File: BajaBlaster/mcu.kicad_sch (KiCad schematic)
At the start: 15 parts, among them J1 Conn_01x06_Socket, SW1 SW_Push, SW2 SW_Push, U1 ESP32-WROOM-32, U2 MPU-6050

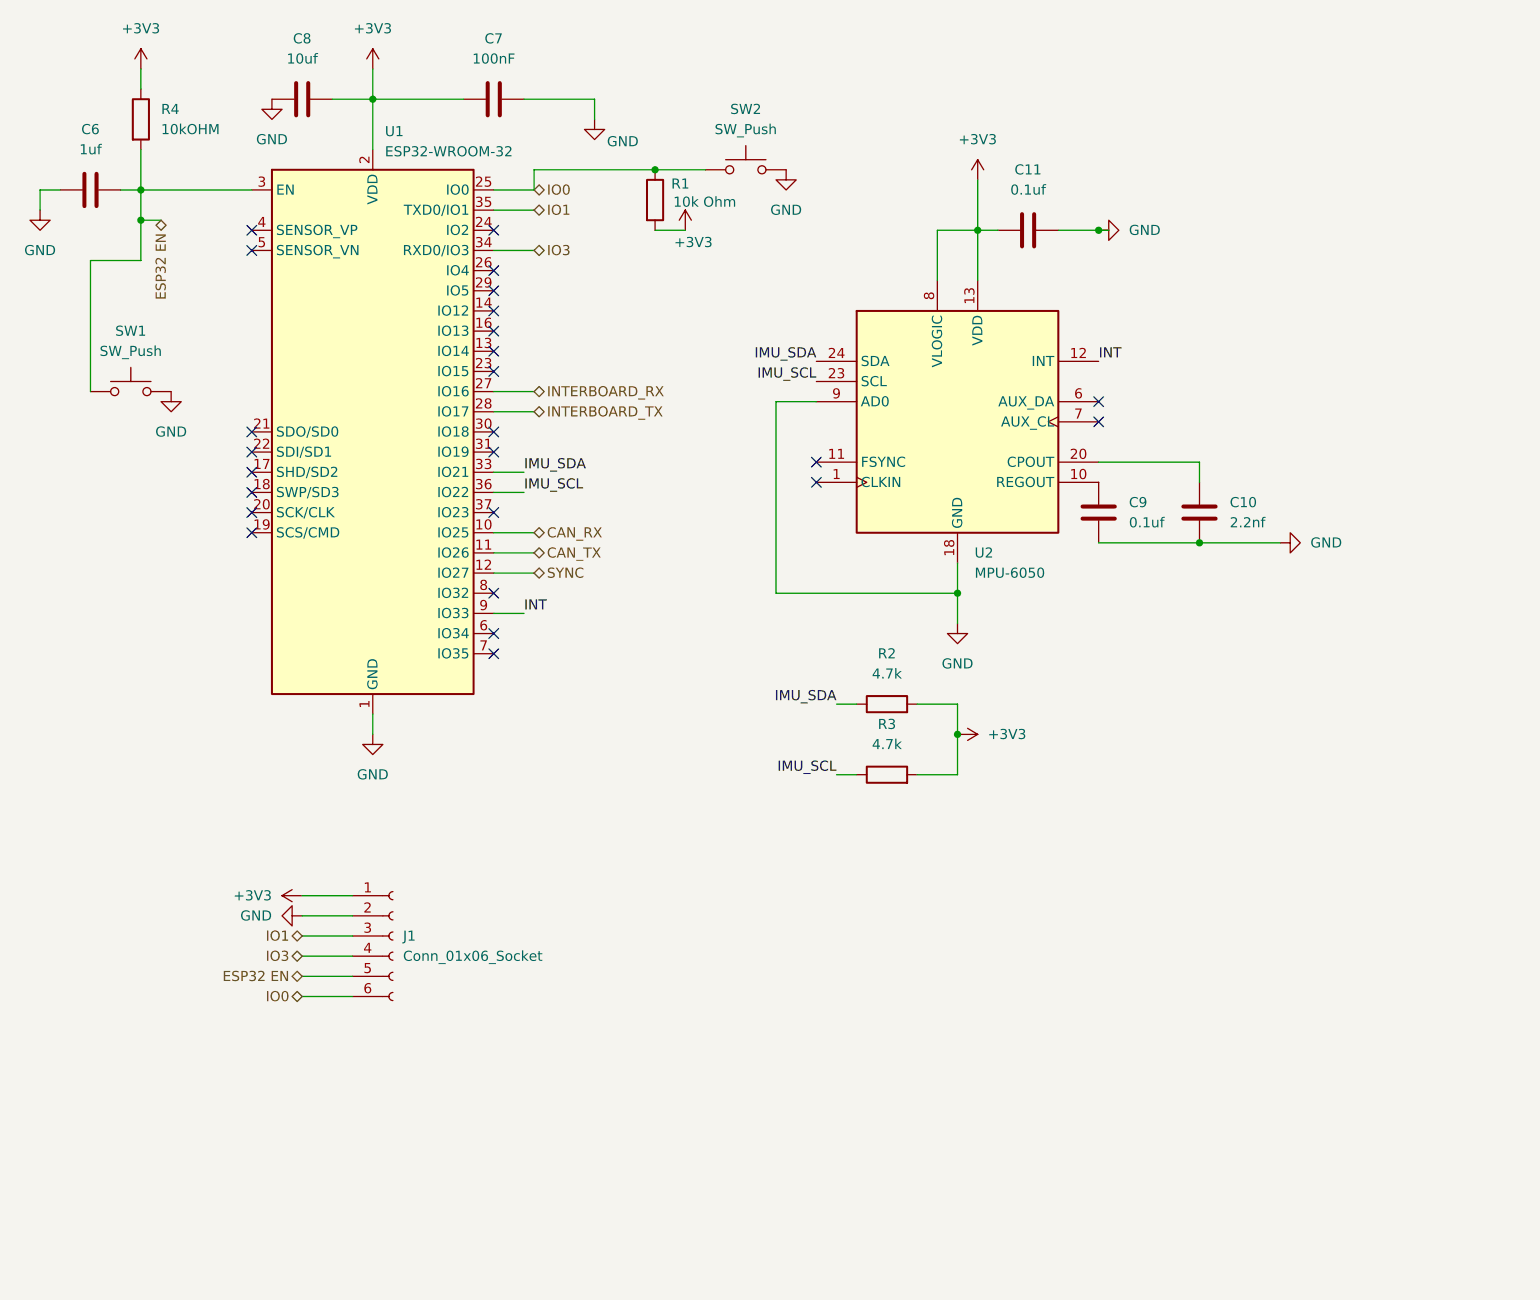
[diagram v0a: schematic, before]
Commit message: doing lots of small tweaks and fixups
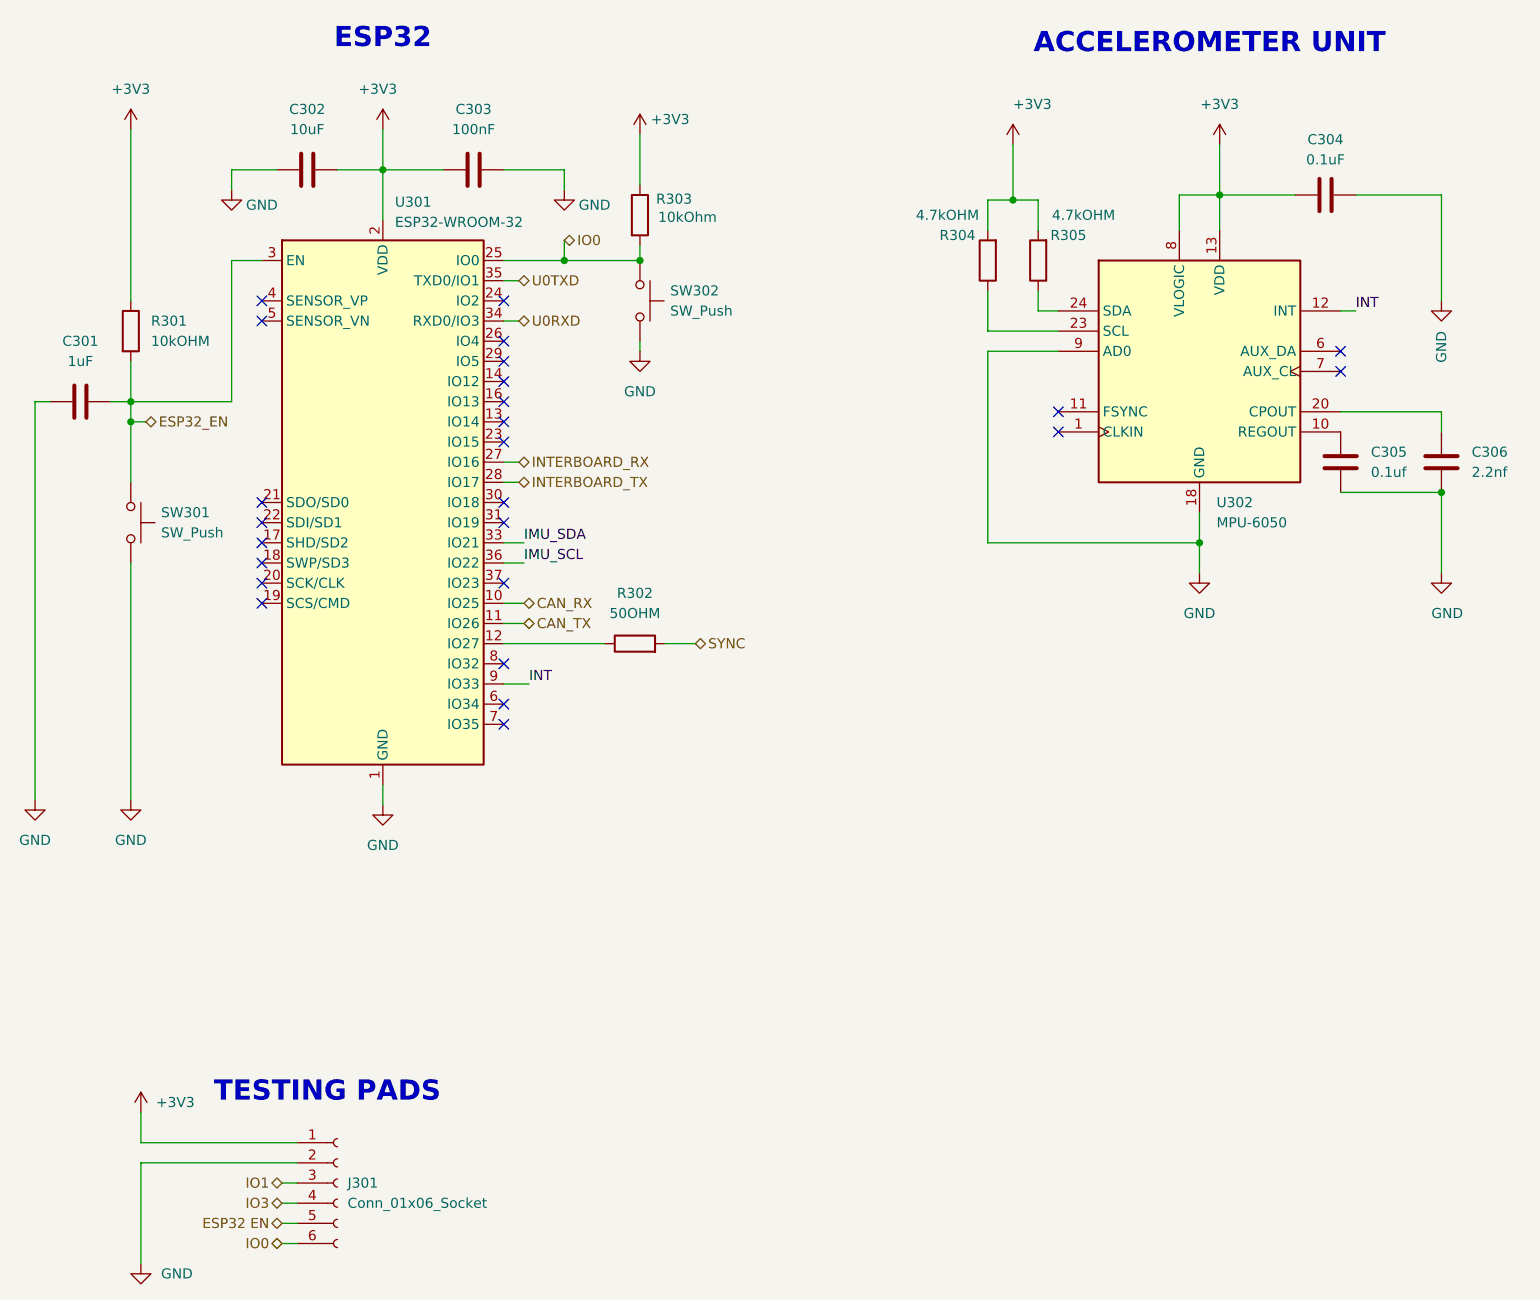
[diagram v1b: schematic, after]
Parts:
- added R302: 50OHM, symbol Device:R
- C301: renamed from C6; value 1uf -> 1uF
- C302: renamed from C8; value 10uf -> 10uF
- C304: renamed from C11; value 0.1uf -> 0.1uF
- R303: renamed from R1; value 10k Ohm -> 10kOhm
- R304: renamed from R2; value 4.7k -> 4.7kOHM
- R305: renamed from R3; value 4.7k -> 4.7kOHM
- renumbered C7 to C303, C9 to C305, C10 to C306, J1 to J301, R4 to R301, SW1 to SW301, SW2 to SW302, U1 to U301, U2 to U302
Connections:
- net +3V3: now also R303.1; no longer R303.2
- net ESP32 EN: no longer C301.1, R301.2, SW301.1, U301.3 (EN)
- net IMU_SCL: no longer R305.1, U302.23 (SCL)
- net IMU_SDA: no longer R304.1, U302.24 (SDA)
- net IO0: now also R303.2; no longer R303.1
- net IO1: no longer U301.35 (TXD0/IO1)
- net IO3: no longer U301.34 (RXD0/IO3)
- net SYNC: now also R302.2; no longer U301.12 (IO27)
- new net: R304.1, U302.23 (SCL)
- new net: R305.1, U302.24 (SDA)
- new net: R302.1, U301.12 (IO27)
- new net ESP32_EN: C301.1, R301.2, SW301.1, U301.3 (EN)
- new net U0RXD: U301.34 (RXD0/IO3)
- new net U0TXD: U301.35 (TXD0/IO1)
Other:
- note added: "ACCELEROMETER UNIT"
- note added: "ESP32"
- note added: "TESTING PADS"
- title: (none) -> MCU_REV_A
- moved on the sheet: C301, C302, C303, C304, C305, C306, J301, R301, R303, R304, R305, SW301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
